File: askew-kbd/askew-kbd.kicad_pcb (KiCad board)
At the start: 2 copper layers, 155.6 x 108.4 mm, 68 parts, among them J1 OLED, J2 MJ-4PP-9, SW1 SW_PUSH, SW10 SW_PUSH, SW11 SW_PUSH, SW12 SW_PUSH, SW13 SW_PUSH, SW14 SW_PUSH, SW15 SW_PUSH, SW16 SW_PUSH, SW17 SW_PUSH, SW18 SW_PUSH, SW19 SW_PUSH, SW2 SW_PUSH, SW20 SW_PUSH, SW21 SW_PUSH, SW22 SW_PUSH, SW3 SW_PUSH, SW4 SW_PUSH, SW5 SW_PUSH, SW6 SW_PUSH, SW7 SW_PUSH, SW8 SW_PUSH, SW9 SW_PUSH, U1 ProMicro

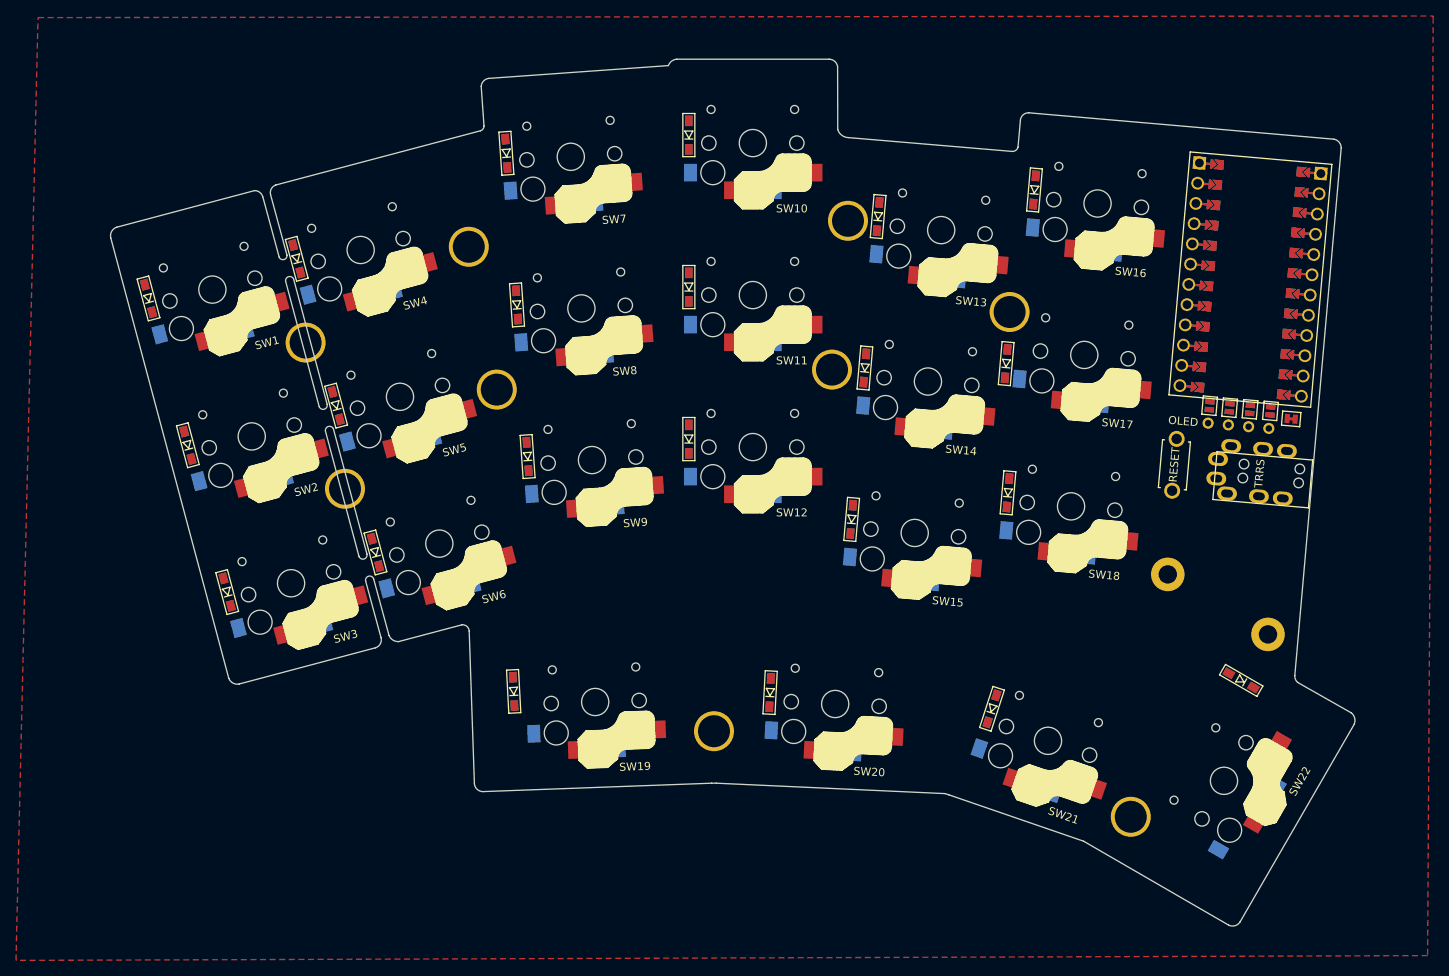
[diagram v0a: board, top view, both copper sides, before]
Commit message: choc_spacing
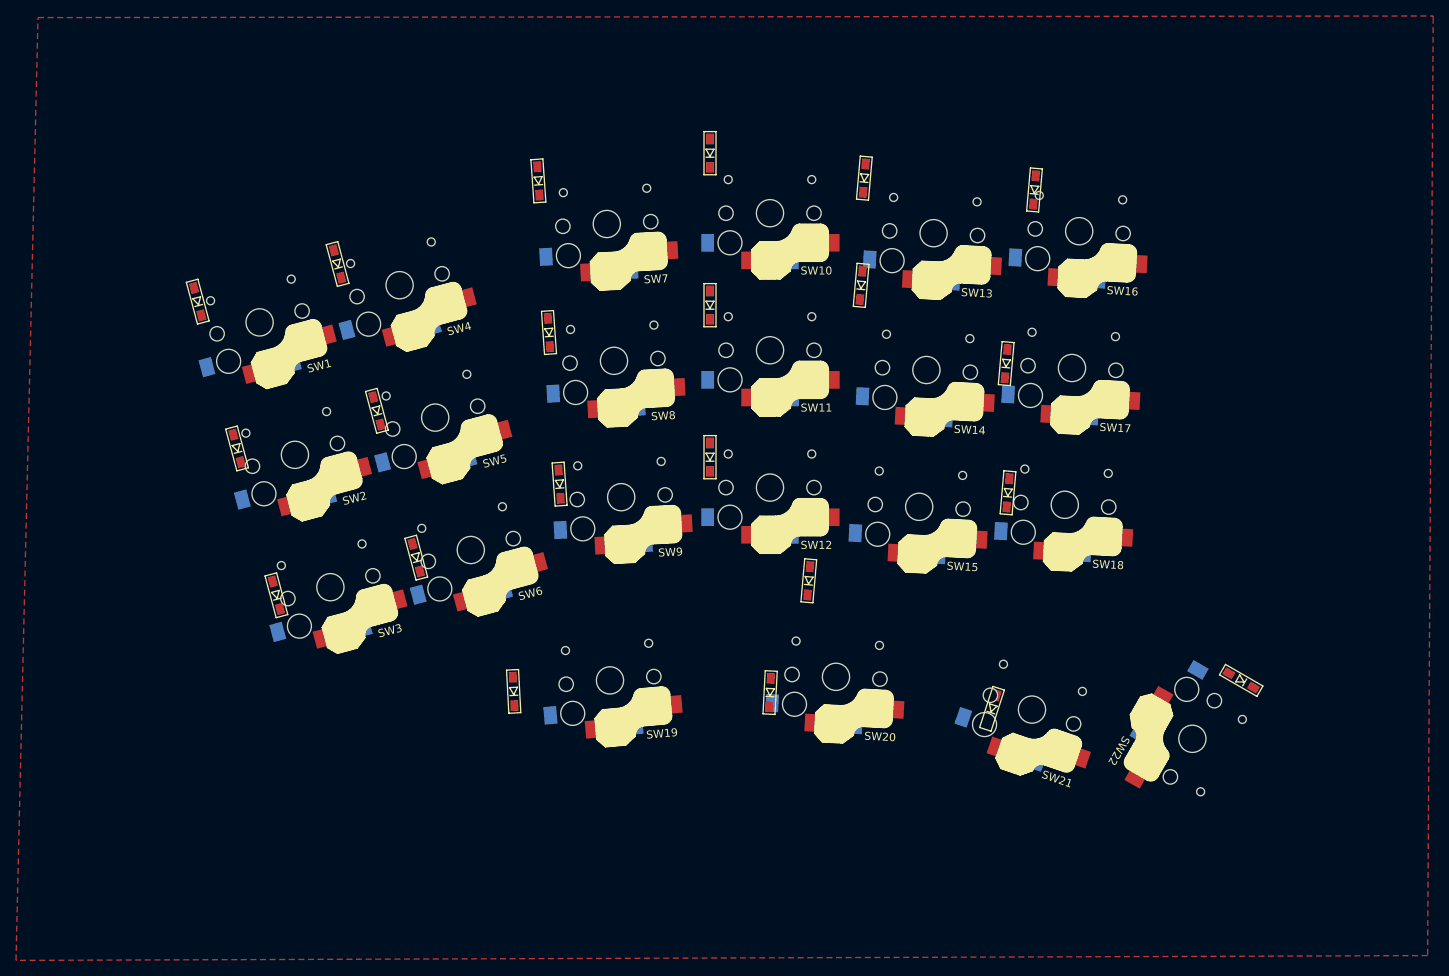
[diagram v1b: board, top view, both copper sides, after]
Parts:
- removed J1: OLED, kbd:OLED_v2
- removed J2: MJ-4PP-9, kbd:MJ-4PP-9
- removed JP1, JP2, JP3, JP4, JP5, JP6, JP7, JP8: , kbd:Jumper
- removed JP9: , kbd:JPC2
- removed REF** (x9): M2_Hole_TH_Outside, kbd:M2_Hole_TH_Outside
- removed REF** (x2): M2_Hole_TH, kbd:M2_Hole_TH
- removed RSW1: SW_PUSH, kbd:ResetSW
- removed U1: ProMicro, keyboard_reversible:ProMicro_unrouted
- SW1, SW10, SW11, SW12, SW13, SW14, SW15, SW16, SW17, SW18, SW2, SW21, SW3, SW4, SW5, SW6, SW7, SW8, SW9: footprint fp:ChocV1_V2_Hotswap_reversed -> fp:ChocV1_V2_Hotswap_reversed_choc_spacing
- SW19, SW20, SW22: footprint fp:ChocV1_V2_Hotswap_reversed_15u -> fp:ChocV1_V2_Hotswap_reversed_15u_choc_spacing
- moved D14 10.3 mm to (154.6, 79.1)
- moved SW7 9.53 mm to (122.8, 71.4), turned to 3 degrees
- moved D15 9.36 mm to (148.1, 116.0)
- moved SW10 9.02 mm to (143.2, 70.0)
- moved SW8 7.71 mm to (123.8, 88.5), turned to 3 degrees
- moved SW11 7.23 mm to (143.3, 87.2)
- moved SW1 7.18 mm to (79.5, 83.7)
- moved SW22 6.57 mm to (196.1, 135.8), turned to -120 degrees
- moved SW4 6.56 mm to (97.0, 79.0)
- moved D2 6.16 mm to (76.6, 99.5)
- moved D3 6.16 mm to (81.5, 117.8)
- moved D1 6.16 mm to (71.7, 81.1)
- moved SW9 5.91 mm to (124.7, 105.5), turned to 3 degrees
- moved SW2 5.87 mm to (83.9, 100.3)
- moved SW12 5.50 mm to (143.2, 104.3)
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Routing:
- net GND: track 0.52 -> 0.00 mm
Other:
- board outline removed
